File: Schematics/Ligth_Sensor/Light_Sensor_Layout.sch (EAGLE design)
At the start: 9 parts, among them J1 RJ45

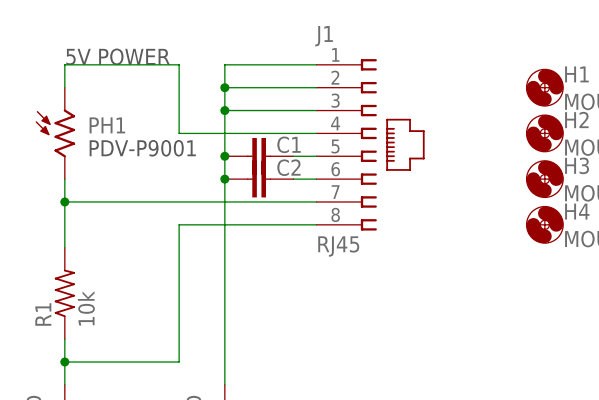
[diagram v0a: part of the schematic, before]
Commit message: Layout for final inspection
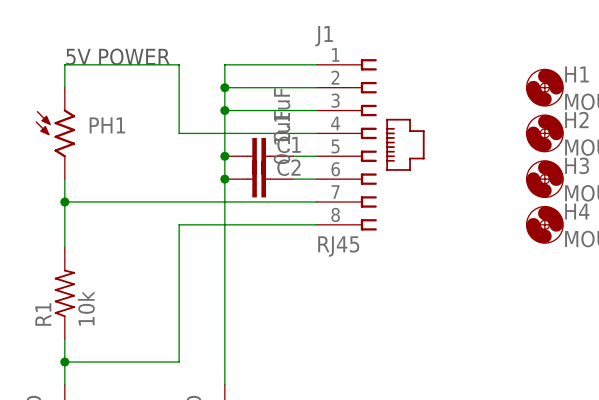
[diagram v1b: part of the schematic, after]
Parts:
- C1, C2: value (none) -> 0.1uF
- PH1: value VT83N2 -> VT90N2; device photo-elements:VT83N2 -> photo-elements:VT90N2
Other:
- note removed: "PDV-P9001"
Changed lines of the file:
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@@
 <?xml version="1.0" encoding="utf-8"?>
 <!DOCTYPE eagle SYSTEM "eagle.dtd">
-<eagle version="6.3">
+<eagle version="6.4">
 <drawing>
 <settings>
@@
 <grid distance="0.1" unitdist="inch" unit="inch" style="lines" multiple="1" display="no" altdistance="0.01" altunitdist="inch" altunit="inch"/>
 <layers>
-<layer number="1" name="Top" color="4" fill="1" visible="yes" active="no"/>
-<layer number="16" name="Bottom" color="1" fill="1" visible="yes" active="no"/>
-<layer number="17" name="Pads" color="2" fill="1" visible="yes" active="no"/>
-<layer number="18" name="Vias" color="2" fill="1" visible="yes" active="no"/>
-<layer number="19" name="Unrouted" color="6" fill="1" visible="yes" active="no"/>
-<layer number="20" name="Dimension" color="15" fill="1" visible="yes" active="no"/>
-<layer number="21" name="tPlace" color="7" fill="1" visible="yes" active="no"/>
-<layer number="22" name="bPlace" color="7" fill="1" visible="yes" active="no"/>
-<layer number="23" name="tOrigins" color="15" fill="1" visible="yes" active="no"/>
-<layer number="24" name="bOrigins" color="15" fill="1" visible="yes" active="no"/>
-<layer number="25" name="tNames" color="7" fill="1" visible="yes" active="no"/>
-<layer number="26" name="bNames" color="7" fill="1" visible="yes" active="no"/>
-<layer number="27" name="tValues" color="7" fill="1" visible="yes" active="no"/>
-<layer number="28" name="bValues" color="7" fill="1" visible="yes" active="no"/>
+<layer number="1" name="Top" color="4" fill="1" visible="no" active="no"/>
+<layer number="16" name="Bottom" color="1" fill="1" visible="no" active="no"/>
+<layer number="17" name="Pads" color="2" fill="1" visible="no" active="no"/>
+<layer number="18" name="Vias" color="2" fill="1" visible="no" active="no"/>
+<layer number="19" name="Unrouted" color="6" fill="1" visible="no" active="no"/>
+<layer number="20" name="Dimension" color="15" fill="1" visible="no" active="no"/>
+<layer number="21" name="tPlace" color="7" fill="1" visible="no" active="no"/>
+<layer number="22" name="bPlace" color="7" fill="1" visible="no" active="no"/>
+<layer number="23" name="tOrigins" color="15" fill="1" visible="no" active="no"/>
+<layer number="24" name="bOrigins" color="15" fill="1" visible="no" active="no"/>
+<layer number="25" name="tNames" color="7" fill="1" visible="no" active="no"/>
+<layer number="26" name="bNames" color="7" fill="1" visible="no" active="no"/>
+<layer number="27" name="tValues" color="7" fill="1" visible="no" active="no"/>
+<layer number="28" name="bValues" color="7" fill="1" visible="no" active="no"/>
 <layer number="29" name="tStop" color="7" fill="3" visible="no" active="no"/>
 <layer number="30" name="bStop" color="7" fill="6" visible="no" active="no"/>
@@
 <layer number="35" name="tGlue" color="7" fill="4" visible="no" active="no"/>
 <layer number="36" name="bGlue" color="7" fill="5" visible="no" active="no"/>
-<layer number="37" name="tTest" color="7" fill="1" visible="yes" active="no"/>
-<layer number="38" name="bTest" color="7" fill="1" visible="yes" active="no"/>
+<layer number="37" name="tTest" color="7" fill="1" visible="no" active="no"/>
+<layer number="38" name="bTest" color="7" fill="1" visible="no" active="no"/>
 <layer number="39" name="tKeepout" color="4" fill="11" visible="no" active="no"/>
 <layer number="40" name="bKeepout" color="1" fill="11" visible="no" active="no"/>
@@
 <layer number="44" name="Drills" color="7" fill="1" visible="no" active="no"/>
 <layer number="45" name="Holes" color="7" fill="1" visible="no" active="no"/>
-<layer number="46" name="Milling" color="3" fill="1" visible="yes" active="no"/>
-<layer number="47" name="Measures" color="7" fill="1" visible="yes" active="no"/>
-<layer number="48" name="Document" color="7" fill="1" visible="yes" active="no"/>
-<layer number="49" name="Reference" color="7" fill="1" visible="yes" active="no"/>
-<layer number="51" name="tDocu" color="7" fill="1" visible="yes" active="no"/>
-<layer number="52" name="bDocu" color="7" fill="1" visible="yes" active="no"/>
+<layer number="46" name="Milling" color="3" fill="1" visible="no" active="no"/>
+<layer number="47" name="Measures" color="7" fill="1" visible="no" active="no"/>
+<layer number="48" name="Document" color="7" fill="1" visible="no" active="no"/>
+<layer number="49" name="Reference" color="7" fill="1" visible="no" active="no"/>
+<layer number="51" name="tDocu" color="7" fill="1" visible="no" active="no"/>
+<layer number="52" name="bDocu" color="7" fill="1" visible="no" active="no"/>
 <layer number="91" name="Nets" color="2" fill="1" visible="yes" active="yes"/>
 <layer number="92" name="Busses" color="1" fill="1" visible="yes" active="yes"/>
@@
 </classes>
 <parts>
-<part name="PH1" library="photo-elements" deviceset="VT8" device="" technology="3N2"/>
+<part name="PH1" library="photo-elements" deviceset="VT9" device="" technology="0N2" value="VT90N2"/>
 <part name="R1" library="rcl" deviceset="R-US_" device="R1206" value="10k"/>
 <part name="J1" library="con-amp" deviceset="555167-1" device="" value="RJ45"/>
@@
 <part name="H4" library="holes" deviceset="MOUNT-HOLE" device="2.8"/>
 <part name="FRAME1" library="frames" deviceset="FRAME_A_L" device="" value="4"/>
-<part name="C1" library="rcl" deviceset="C-EU" device="C0603K"/>
-<part name="C2" library="rcl" deviceset="C-EU" device="C0603K"/>
+<part name="C1" library="rcl" deviceset="C-EU" device="C0603K" value="0.1uF"/>
+<part name="C2" library="rcl" deviceset="C-EU" device="C0603K" value="0.1uF"/>
 </parts>
 <sheets>
 <sheet>
 <plain>
-<text x="88.9" y="53.34" size="1.778" layer="97">PDV-P9001</text>
 <text x="86.36" y="63.5" size="1.778" layer="97">5V POWER</text>
 <text x="149.86" y="-20.32" size="2.54" layer="94">LIGHT SENSOR BOARD</text>
